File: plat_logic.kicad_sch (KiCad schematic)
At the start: 63 parts, among them SW1 Button-SMD-4.5x4.5x5.5, SW2 Button-SMD-4.5x4.5x5.5, U2 USBLC6-2SC6, U2.1 STM32F429ZIT6TR_split, U2.2 STM32F429ZIT6TR_split, U2.3 STM32F429ZIT6TR_split, U2.4 STM32F429ZIT6TR_split, X1 NX3225GD 8.000MHZ EXS00A-CG06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, X2 NX3215SA-32.768KHZ-EXS00A-MU0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

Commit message: footprints, symbols kicad
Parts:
- removed C1: 2pF, symbol 0805_C9900012713_2
- removed C2: 2pF, symbol 0805_C9900012713_3
- removed C3: 2pF, symbol 0805_C9900012713
- removed C39, C40: 50pF, symbol Device:C
- removed C4: 2pF, symbol 0805_C9900012713_1
- removed C5, C61: 100nF, symbol 0805_C9900012713_6
- removed C6: 1uF x5r, symbol C_0603_US
- removed C7: 2.2uF_x7r, symbol 0805_C9900012713_5
- removed C8: 2.2uF_x7r, symbol 0805_C9900012713_4
- removed Con1: (no value), symbol MyLIB:Con
- removed D26: BAS70, symbol SS54L_19
- removed JP1, JP2: Jumper_2_Open, symbol Jumper:Jumper_2_Open
- removed L1: 1m, symbol L0603_US
- removed R1: 0Ω, symbol RMC1/8JPTP
- removed R10: 0, symbol R_0603_EU_3
- removed R2: 0Ω, symbol RMC1/8JPTP_1
- removed R3: 0, symbol R_0603_EU_6
- removed R39, R41: 25K, symbol Device:R
- removed R4: 0, symbol R_0603_EU_1
- removed R40: 10K, symbol Device:R
- removed R45: 1k, symbol Device:R
- removed R5: 0, symbol R_0603_EU_5
- removed R6: 0, symbol R_0603_EU_4
- removed R63, R64, R65, R66: 2.2k, symbol Device:R
- removed R7: 0, symbol R_0603_EU
- removed R8: 10K, symbol R_0603_EU_7
- removed R9: 0, symbol R_0603_EU_2
- removed SW1, SW2: Button-SMD-4.5x4.5x5.5, symbol Button-SMD-4.5x4.5x5.5
- removed U2: USBLC6-2SC6, Package_TO_SOT_SMD:SOT-23-6, symbol Power_Protection:USBLC6-2SC6
- removed U2.1: STM32F429ZIT6TR_split, symbol STM32F429ZIT6TR_split
- removed U2.2: STM32F429ZIT6TR_split, symbol STM32F429ZIT6TR_split_1
- removed U2.3: STM32F429ZIT6TR_split, symbol STM32F429ZIT6TR_split_2
- removed U2.4: STM32F429ZIT6TR_split, symbol STM32F429ZIT6TR_split_3
- removed X1: NX3225GD 8.000MHZ EXS00A-CG06684, symbol NX3225GD 8.000MHZ EXS00A-CG06684
- removed X2: NX3215SA-32.768KHZ-EXS00A-MU00746, symbol NX3215SA-32.768KHZ-EXS00A-MU00746
- added C10: 1uF_x7r, Capacitor_SMD:C_0603_1608Metric, symbol 0805_C9900012713_5
- added C11: 1uF_x7r, Capacitor_SMD:C_0603_1608Metric, symbol 0805_C9900012713_4
- added C12, C62: 100nF, Capacitor_SMD:C_0402_1005Metric, symbol 0805_C9900012713_6
- added C13: 12pF, Capacitor_SMD:C_0603_1608Metric, symbol 0805_C9900012713_2
- added C14: 12pF, Capacitor_SMD:C_0603_1608Metric, symbol 0805_C9900012713_3
- added C15: 12pF, Capacitor_SMD:C_0603_1608Metric, symbol 0805_C9900012713
- added C16: 12pF, Capacitor_SMD:C_0603_1608Metric, symbol 0805_C9900012713_1
- added C45, C46: 22pF, Capacitor_SMD:C_0603_1608Metric, symbol Device:C
- added C9: 1uF x5r, Capacitor_SMD:C_0603_1608Metric, symbol C_0603_US
- added D28: BAS70, Package_TO_SOT_SMD:SOT-23, symbol SS54L_19
- added JP3, JP4: Jumper_2_Open, Jumper:SolderJumper-2_P1.3mm_Open_Pad1.0x1.5mm, symbol Jumper:Jumper_2_Open
- added L2: 1m, symbol L0603_US
- added R14: 0, symbol R_0603_EU
- added R15: 0, symbol R_0603_EU_1
- added R16: 0, symbol R_0603_EU_6
- added R17: 0, symbol R_0603_EU_5
- added R18: 0, symbol R_0603_EU_4
- added R19: 0, symbol R_0603_EU_2
- added R20: 0, symbol R_0603_EU_3
- added R21: 10K, Resistor_SMD:R_0201_0603Metric, symbol R_0603_EU_7
- added R22: 0Ω, symbol RMC1/8JPTP
- added R35: 0Ω, symbol RMC1/8JPTP_1
- added R49: 1k, Resistor_SMD:R_0805_2012Metric, symbol Device:R
- added R50, R57: 27K, Resistor_SMD:R_0805_2012Metric, symbol Device:R
- added R58: 10K, Resistor_SMD:R_0201_0603Metric, symbol Device:R
- added R67, R68, R69, R70: 2.2k, Resistor_SMD:R_0805_2012Metric, symbol Device:R
- added SW3, SW4: Button-SMD-4.5x4.5x5.5, Button_Switch_SMD:SW_SPST_PTS647_Sx50, symbol Button-SMD-4.5x4.5x5.5
- added U1: STM32F429ZITx, Package_QFP:LQFP-144_20x20mm_P0.5mm, symbol MCU_ST_STM32F4:STM32F429ZITx
- added U3: USBLC6-2SC6, Package_TO_SOT_SMD:SOT-23-6, symbol Power_Protection:USBLC6-2SC6
- added X3: NX3225GD 8.000MHZ EXS00A-CG06684, Crystal:Crystal_SMD_3225-4Pin_3.2x2.5mm, symbol NX3225GD 8.000MHZ EXS00A-CG06684
- added X4: NX3215SA-32.768KHZ-EXS00A-MU00746, Crystal:Crystal_SMD_3215-2Pin_3.2x1.5mm, symbol NX3215SA-32.768KHZ-EXS00A-MU00746
- C42: footprint (none) -> Capacitor_SMD:C_0603_1608Metric
- C47, C48, C49, C50, C51, C52: footprint (none) -> Capacitor_SMD:C_0402_1005Metric
- D27: footprint (none) -> Package_SO:VSSOP-8_2.3x2mm_P0.5mm
- R11: footprint (none) -> Resistor_SMD:R_0805_2012Metric
- R46, R47, R48: footprint (none) -> Resistor_SMD:R_0201_0603Metric
- R51, R52, R53, R54, R55, R56: value 50 -> 47; footprint (none) -> Resistor_SMD:R_0805_2012Metric
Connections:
- net +3v3: now also D28.1 (K), JP3.2 (B), JP4.1 (A), L2.1, R15.1, R18.1, R19.2, R58.2, R67.1, R68.1, R69.1, R70.1, U1.108 (VDD), U1.121 (VDD), U1.131 (VDD), U1.144 (VDD), U1.17 (VDD), U1.30 (VDD), U1.39 (VDD), U1.52 (VDD), U1.62 (VDD), U1.72 (VDD), U1.84 (VDD), U1.95 (VDD)
- net +5v: now also U3.5 (VBUS)
- net A0: now also U1.141 (PE0)
- net A1: now also U1.142 (PE1)
- net A2: now also U1.1 (PE2)
- net A3: now also U1.2 (PE3)
- net A4: now also U1.3 (PE4)
- net A5: now also U1.4 (PE5)
- net A6: now also U1.5 (PE6)
- net A7: now also U1.63 (PE10)
- net AGND: now also U1.31 (VSSA)
- net BOOT0: now also JP3.1 (A), R21.1, U1.138 (BOOT0)
- net BOOT1: now also JP4.2 (B), U1.48 (PB2)
- net D10: now also U1.77 (PD8)
- net D11: now also U1.79 (PD10)
- net D12: now also U1.80 (PD11)
- net D13: now also U1.135 (PB5)
- net D2: now also U1.114 (PD0)
- net D3: now also U1.115 (PD1)
- net D4: now also U1.116 (PD2)
- net D5: now also U1.117 (PD3)
- net D6: now also U1.118 (PD4)
- net D7: now also U1.119 (PD5)
- net D8: now also U1.122 (PD6)
- net D9: now also U1.123 (PD7)
- net DAC(PA4): now also C45.1, R50.1, U1.40 (PA4)
- net DAC(PA5): now also C46.1, R57.1, U1.41 (PA5)
- net ENC_A_M1: now also U1.55 (PF15)
- net ENC_A_M2: now also U1.53 (PF13)
- net ENC_A_M3: now also U1.59 (PE8)
- net ENC_A_M4: now also U1.57 (PG1)
- net ENC_A_M5: now also R67.2, U1.96 (PC6)
- net ENC_A_M6: now also R69.2, U1.81 (PD12)
- net ENC_B_M1: now also U1.56 (PG0)
- net ENC_B_M2: now also U1.54 (PF14)
- net ENC_B_M3: now also U1.60 (PE9)
- net ENC_B_M4: now also U1.58 (PE7)
- net ENC_B_M5: now also R68.2, U1.97 (PC7)
- net ENC_B_M6: now also R70.2, U1.82 (PD13)
- net GND: now also C10.2, C11.1, C12.2, C13.1, C14.1, C15.2, C16.2, C45.2, C46.2, C62.2, C9.2, R16.2, R20.2, R21.2, R50.2, R57.2, SW3.3, SW3.4, SW4.3, SW4.4, U1.107 (VSS), U1.120 (VSS), U1.130 (VSS), U1.16 (VSS), U1.38 (VSS), U1.51 (VSS), U1.61 (VSS), U1.83 (VSS), U1.94 (VSS), U3.2 (GND)
- net I2C2_SCL: now also U1.11 (PF1)
- net I2C2_SDA: now also U1.10 (PF0)
- net I2C_SCL: now also U1.139 (PB8)
- net I2C_SDA: now also U1.140 (PB9)
- net NRST: now also D28.2 (A), R58.1, SW4.1, U1.25 (NRST)
- net PA15: now also U1.110 (PA15)
- net PA2: now also U1.36 (PA2)
- net PA3: now also U1.37 (PA3)
- net PA6: now also U1.42 (PA6)
- net PA7: now also U1.43 (PA7)
- net PC0: now also U1.26 (PC0)
- net PC1: now also U1.27 (PC1)
- net PC3(A2): now also U1.29 (PC3)
- net PF10(A5): now also U1.22 (PF10)
- net PF3(A3): now also U1.13 (PF3)
- net PF5(A4): now also U1.15 (PF5)
- net PG13: now also U1.128 (PG13)
- net PG14: now also U1.129 (PG14)
- net PH2: now also R17.1
- net SWO: now also U1.133 (PB3)
- net TCK: now also U1.109 (PA14)
- net TMS: now also U1.105 (PA13)
- net TX_Enable(Dynamixel_TTL): now also U1.113 (PC12)
- net USART4_RX(Dynamixel_TTL): now also U1.112 (PC11)
- net USART4_TX: now also U1.34 (PA0)
- net USART4_TX(Dynamixel_TTL): now also U1.111 (PC10)
- net VBUS(PA9): now also R49.2
- net ext_RXD: now also U1.69 (PB10)
- net ext_TXD: now also U1.78 (PD9)
- net extra1_enc_A: now also U1.85 (PD14)
- net extra1_enc_B: now also U1.86 (PD15)
- net extra2_enc_A: now also U1.87 (PG2)
- net extra2_enc_B: now also U1.88 (PG3)
- new net: R49.1, U1.101 (PA9)
- new net: U1.103 (PA11), U3.3 (I/O2)
- new net: U1.104 (PA12), U3.1 (I/O1)
- new net: C11.2, R17.2, R18.2, U1.106 (VCAP_2)
- new net: SW3.1, U1.127 (PG12)
- new net: R19.1, R20.1, U1.143 (PDR_ON)
- new net: C9.1, R15.2, U1.6 (VBAT)
- new net: C10.1, R16.1, U1.71 (VCAP_1)
- new net: C13.2, R22.1, X3.1
- new net: C14.2, R35.1, X3.2 (GND)
- new net: L2.2, R14.1
- new net: C12.1, SW4.2
- new net: C62.1, SW3.2
- new net PC14: C15.1, U1.8 (PC14), X4.1 (OSC1)
- new net PC15: C16.1, U1.9 (PC15), X4.2 (OSC2)
- new net PH0: R22.2, U1.23 (PH0)
- new net PH1: R35.2, U1.24 (PH1)
- new net USBDM(PA12): U3.6 (I/O1)
- new net USBDP(PA11): U3.4 (I/O2)
- new net VDDA: R14.2, U1.32 (VREF+), U1.33 (VDDA)
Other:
- moved on the sheet: C42, C47, C48, C49, C50, C51, C52, D27, R11, R12, R13, R46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

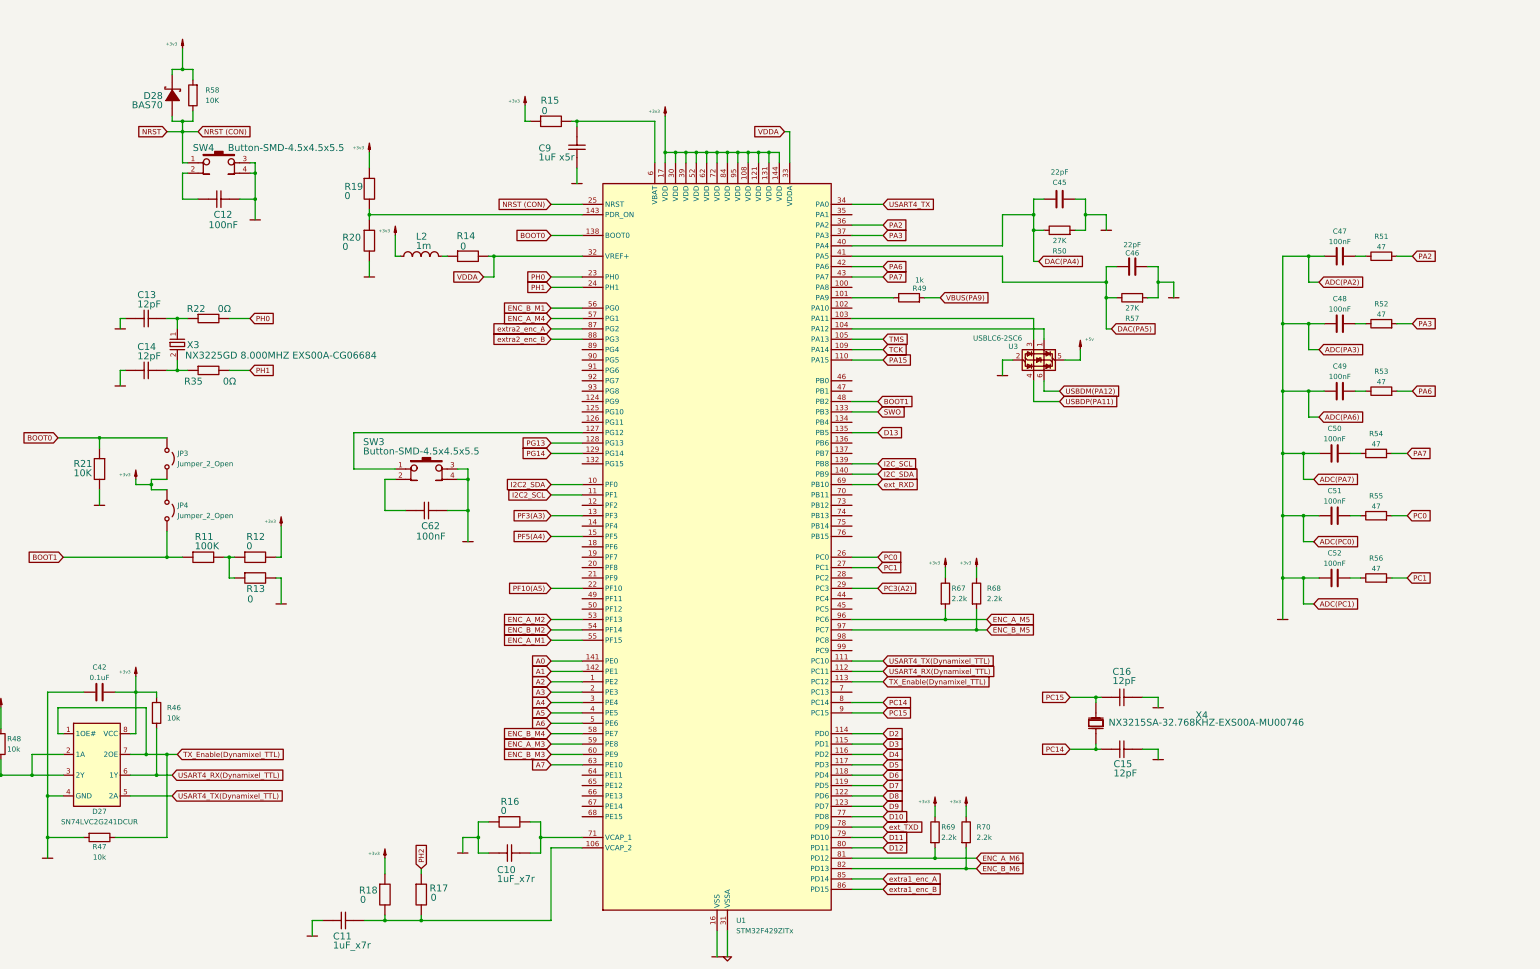
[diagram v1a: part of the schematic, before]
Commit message: Add files via upload
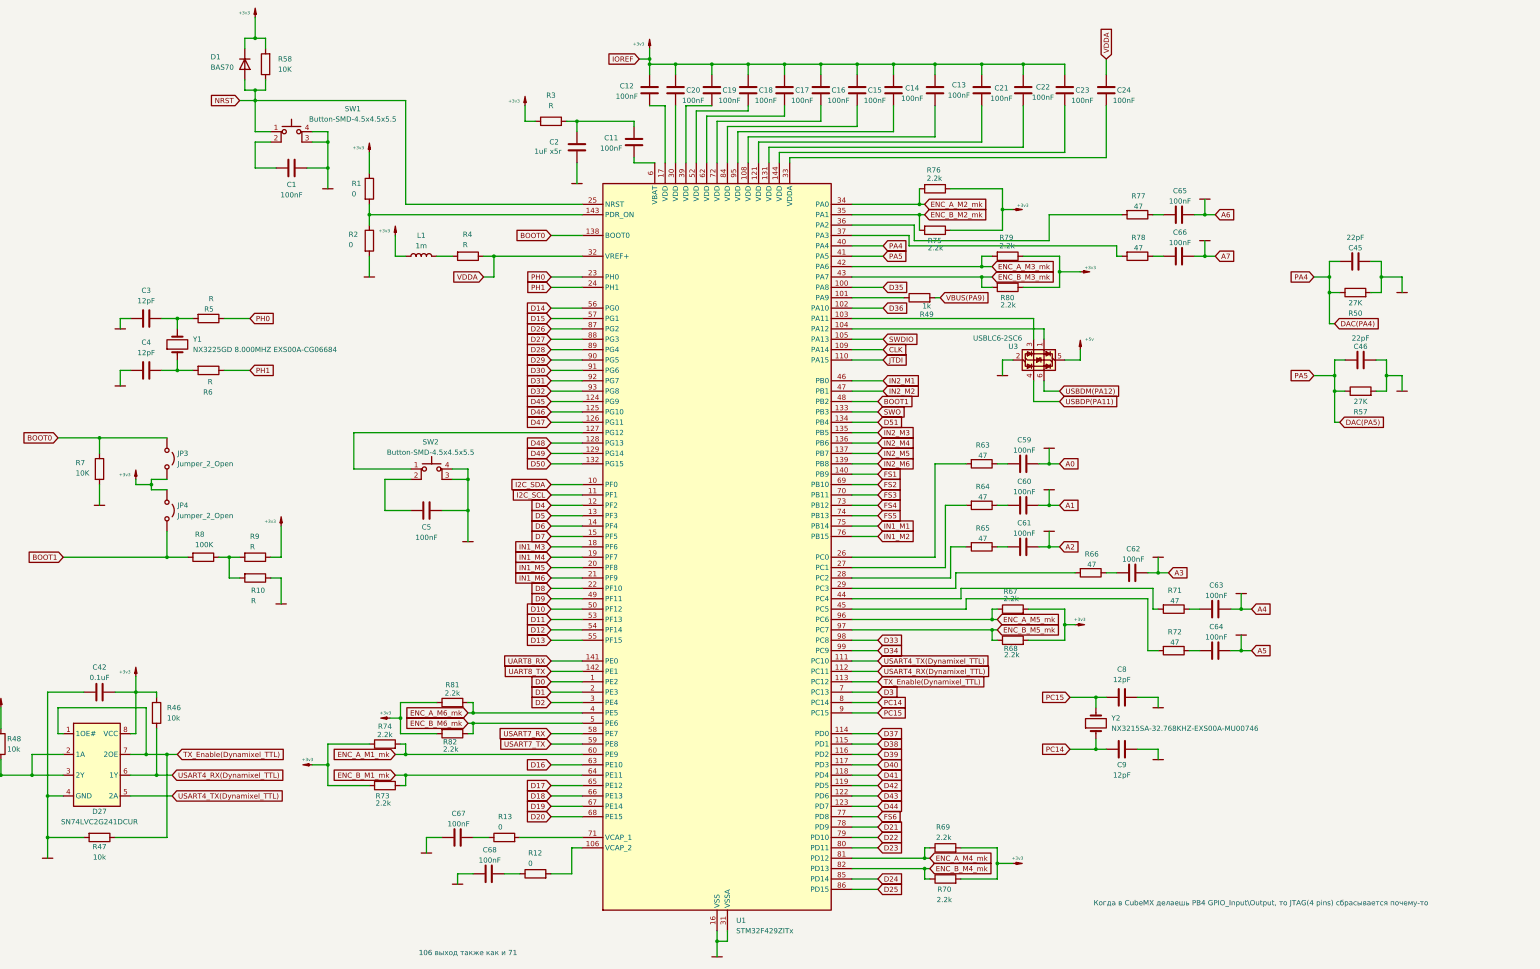
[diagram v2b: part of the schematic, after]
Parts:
- removed C10: 1uF_x7r, Capacitor_SMD:C_0603_1608Metric, symbol 0805_C9900012713_5
- removed C11: 1uF_x7r, Capacitor_SMD:C_0603_1608Metric, symbol 0805_C9900012713_4
- removed C12, C62: 100nF, Capacitor_SMD:C_0402_1005Metric, symbol 0805_C9900012713_6
- removed C13: 12pF, Capacitor_SMD:C_0603_1608Metric, symbol 0805_C9900012713_2
- removed C14: 12pF, Capacitor_SMD:C_0603_1608Metric, symbol 0805_C9900012713_3
- removed C15: 12pF, Capacitor_SMD:C_0603_1608Metric, symbol 0805_C9900012713
- removed C16: 12pF, Capacitor_SMD:C_0603_1608Metric, symbol 0805_C9900012713_1
- removed C47, C48, C49, C50, C51, C52: 100nF, Capacitor_SMD:C_0402_1005Metric, symbol Device:C
- removed C9: 1uF x5r, Capacitor_SMD:C_0603_1608Metric, symbol C_0603_US
- removed D28: BAS70, Package_TO_SOT_SMD:SOT-23, symbol SS54L_19
- removed L2: 1m, symbol L0603_US
- removed R11: 100K, Resistor_SMD:R_0805_2012Metric, symbol R_0603_EU_8
- removed R12: 0, symbol R_0603_EU_9
- removed R13: 0, symbol R_0603_EU_10
- removed R14: 0, symbol R_0603_EU
- removed R15: 0, symbol R_0603_EU_1
- removed R16: 0, symbol R_0603_EU_6
- removed R17: 0, symbol R_0603_EU_5
- removed R18: 0, symbol R_0603_EU_4
- removed R19: 0, symbol R_0603_EU_2
- removed R20: 0, symbol R_0603_EU_3
- removed R21: 10K, Resistor_SMD:R_0201_0603Metric, symbol R_0603_EU_7
- removed R22: 0Ω, symbol RMC1/8JPTP
- removed R35: 0Ω, symbol RMC1/8JPTP_1
- removed R51, R52, R53, R54, R55, R56: 47, Resistor_SMD:R_0805_2012Metric, symbol Device:R
- removed SW3, SW4: Button-SMD-4.5x4.5x5.5, Button_Switch_SMD:SW_SPST_PTS647_Sx50, symbol Button-SMD-4.5x4.5x5.5
- removed X3: NX3225GD 8.000MHZ EXS00A-CG06684, Crystal:Crystal_SMD_3225-4Pin_3.2x2.5mm, symbol NX3225GD 8.000MHZ EXS00A-CG06684
- removed X4: NX3215SA-32.768KHZ-EXS00A-MU00746, Crystal:Crystal_SMD_3215-2Pin_3.2x1.5mm, symbol NX3215SA-32.768KHZ-EXS00A-MU00746
- added C1, C11, C12, C13, C14, C15, C16, C17, C18, C19, C20, C21, C22, C23, C24: 100nF, Capacitor_SMD:C_0603_1608Metric, symbol Device:C
- added C2: 1uF x5r, Capacitor_SMD:C_0603_1608Metric, symbol Device:C
- added C3, C4, C8, C9: 12pF, Capacitor_SMD:C_0603_1608Metric, symbol Device:C
- added C5, C59, C60, C61, C62, C63, C64, C65, C66, C67, C68: 100nF, Capacitor_SMD:C_0402_1005Metric, symbol Device:C
- added D1: BAS70, Diode_SMD:D_0603_1608Metric, symbol Diode:1N914
- added L1: 1m, symbol Device:L
- added R1, R12, R13, R2: 0, Resistor_SMD:R_0805_2012Metric, symbol Device:R
- added R10, R3, R4, R5, R6, R9: R, symbol Device:R
- added R63, R64, R65, R66, R71, R72, R77, R78: 47, Resistor_SMD:R_0805_2012Metric, symbol Device:R
- added R7: 10K, Resistor_SMD:R_0201_0603Metric, symbol Device:R
- added R73, R74, R75, R76, R79, R80, R81, R82: 2.2k, Resistor_SMD:R_0805_2012Metric, symbol Device:R
- added R8: 100K, Resistor_SMD:R_0805_2012Metric, symbol Device:R
- added SW1, SW2: Button-SMD-4.5x4.5x5.5, Button_Switch_SMD:SW_SPST_PTS647_Sx50, symbol Switch:SW_MEC_5E
- added Y1: NX3225GD 8.000MHZ EXS00A-CG06684, Crystal:Crystal_SMD_3225-4Pin_3.2x2.5mm, symbol Device:Crystal
- added Y2: NX3215SA-32.768KHZ-EXS00A-MU00746, Crystal:Crystal_SMD_3215-2Pin_3.2x1.5mm, symbol Device:Crystal
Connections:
- net A4 is gone; now on net D2: U1.3 (PE4)
- net AGND is gone; now on net GND: U1.31 (VSSA)
- net ENC_A_M1 is gone; now on net D13: U1.55 (PF15)
- net ENC_A_M2 is gone; now on net D11: U1.53 (PF13)
- net ENC_B_M2 is gone; now on net D12: U1.54 (PF14)
- net I2C2_SCL is gone; now on net I2C_SCL: U1.11 (PF1)
- net I2C2_SDA is gone; now on net I2C_SDA: U1.10 (PF0)
- net PF10(A5) is gone; now on net D8: U1.22 (PF10)
- net PF3(A3) is gone; now on net D5: U1.13 (PF3)
- net PF5(A4) is gone; now on net D7: U1.15 (PF5)
- net +3v3: now also R67.2, R68.2, R69.2, R70.2, C12.1, C13.1, C14.1, C15.1, C16.1, C17.1, C18.1, C19.1, C20.1, C21.1, C22.1, C23.1, D1.1 (K), L1.1, R1.1, R3.1, R73.2, R74.1, R75.1, R76.1, R79.1, R80.1, R81.1, R82.2, R9.1; no longer R67.1, R68.1, R69.1, R70.1, U1.108 (VDD), U1.121 (VDD), U1.131 (VDD), U1.144 (VDD), U1.17 (VDD), U1.30 (VDD), U1.39 (VDD), U1.52 (VDD), U1.62 (VDD), U1.72 (VDD), U1.84 (VDD), U1.95 (VDD)
- net BOOT0: now also R7.1
- net BOOT1: now also R8.2
- net D10: now also U1.50 (PF12); no longer U1.77 (PD8)
- net D11: no longer U1.79 (PD10)
- net D12: no longer U1.80 (PD11)
- net D13: no longer U1.135 (PB5)
- net D2: no longer U1.114 (PD0)
- net D3: now also U1.7 (PC13); no longer U1.115 (PD1)
- net D4: now also U1.12 (PF2); no longer U1.116 (PD2)
- net D5: no longer U1.117 (PD3)
- net D6: now also U1.14 (PF4); no longer U1.118 (PD4)
- net D7: no longer U1.119 (PD5)
- net D8: no longer U1.122 (PD6)
- net D9: now also U1.49 (PF11); no longer U1.123 (PD7)
- net GND: now also C1.2, C2.1, C3.1, C4.1, C5.2, C59.2, C60.2, C61.2, C62.2, C63.2, C64.2, C65.2, C66.2, C67.1, C68.1, C8.2, C9.2, R10.1, R2.2, R7.2, SW1.3 (K), SW1.4 (A), SW2.3 (K), SW2.4 (A)
- net I2C_SCL: no longer U1.139 (PB8)
- net I2C_SDA: no longer U1.140 (PB9)
- net NRST: now also D1.2 (A), SW1.1
- net PC14: now also C9.1, Y2.1
- net PC15: now also C8.1, Y2.2
- net PH0: now also R5.1
- net PH1: now also R6.1
- net VDDA: now also C24.1, R4.1; no longer U1.33 (VDDA)
- net D35: now reaches U1.100 (PA8)
- net D36: now reaches U1.102 (PA10)
- net at U1.106 (VCAP_2): now also R12.2
- net D45: now reaches U1.124 (PG9)
- net D46: now reaches U1.125 (PG10)
- net D47: now reaches U1.126 (PG11)
- net at U1.127 (PG12): now also SW2.1
- net D50: now reaches U1.132 (PG15)
- net D51: now reaches U1.134 (PB4)
- net IN2_M4: now reaches U1.136 (PB6)
- net IN2_M5: now reaches U1.137 (PB7)
- net at U1.143 (PDR_ON): now also R1.2, R2.1
- net IN1_M3: now reaches U1.18 (PF6)
- net IN1_M4: now reaches U1.19 (PF7)
- net IN1_M5: now reaches U1.20 (PF8)
- net IN1_M6: now reaches U1.21 (PF9)
- net at U1.28 (PC2): now also R65.2
- net ENC_B_M2_mk: now reaches U1.35 (PA1)
- net ENC_B_M2_mk: now also R75.2
- net at U1.44 (PC4): now also R71.2
- net at U1.45 (PC5): now also R72.2
- net IN2_M1: now reaches U1.46 (PB0)
- net IN2_M2: now reaches U1.47 (PB1)
- net at U1.6 (VBAT): now also C11.2
- net ENC_B_M1_mk: now reaches U1.64 (PE11)
- net ENC_B_M1_mk: now also R73.1
- net D17: now reaches U1.65 (PE12)
- net D18: now reaches U1.66 (PE13)
- net D19: now reaches U1.67 (PE14)
- net D20: now reaches U1.68 (PE15)
- net FS3: now reaches U1.70 (PB11)
- net at U1.71 (VCAP_1): now also R13.2
- net FS4: now reaches U1.73 (PB12)
- net FS5: now reaches U1.74 (PB13)
- net IN1_M1: now reaches U1.75 (PB14)
- net IN1_M2: now reaches U1.76 (PB15)
- net D28: now reaches U1.89 (PG4)
- net D29: now reaches U1.90 (PG5)
- net D30: now reaches U1.91 (PG6)
- net D31: now reaches U1.92 (PG7)
- net D32: now reaches U1.93 (PG8)
- net D33: now reaches U1.98 (PC8)
- net D34: now reaches U1.99 (PC9)
- net A0 renamed UART8_RX
- net A1 renamed UART8_TX
- net A2 renamed D0
- net A3 renamed D1
- net A5 renamed ENC_A_M6_mk
- net ENC_A_M6_mk: now also R81.2
- net A6 renamed ENC_B_M6_mk
- net ENC_B_M6_mk: now also R82.1
- net A7 renamed D16
- net ENC_A_M3 renamed USART7_TX
- net ENC_A_M4 renamed D15
- net ENC_A_M5 renamed ENC_A_M5_mk
- net ENC_A_M5_mk: now also R67.1; no longer R67.2
- net ENC_A_M6 renamed ENC_A_M4_mk
- net ENC_A_M4_mk: now also R69.1; no longer R69.2
- net ENC_B_M1 renamed D14
- net ENC_B_M3 renamed ENC_A_M1_mk
- net ENC_A_M1_mk: now also R74.2
- net ENC_B_M4 renamed USART7_RX
- net ENC_B_M5 renamed ENC_B_M5_mk
- net ENC_B_M5_mk: now also R68.1; no longer R68.2
- net ENC_B_M6 renamed ENC_B_M4_mk
- net ENC_B_M4_mk: now also R70.1; no longer R70.2
- net PA15 renamed JTDI
- net PA2: no longer names the net of U1.36 (PA2)
- net PA2: now also R77.2
- net PA3: no longer names the net of U1.37 (PA3)
- net PA3: now also R78.2
- net PA6 renamed ENC_A_M3_mk
- net ENC_A_M3_mk: now also R79.2
- net PA7 renamed ENC_B_M3_mk
- net ENC_B_M3_mk: now also R80.2
- net PC0: no longer names the net of U1.26 (PC0)
- net PC0: now also R63.2
- net PC1: no longer names the net of U1.27 (PC1)
- net PC1: now also R64.2
- net PC3(A2): no longer names the net of U1.29 (PC3)
- net PC3(A2): now also R66.2
- net PG13 renamed D48
- net PG14 renamed D49
- net TCK renamed CLK
- net TMS renamed SWDIO
- net USART4_TX renamed ENC_A_M2_mk
- net ENC_A_M2_mk: now also R76.2
- net ext_RXD renamed FS2
- net ext_TXD renamed D21
- net extra1_enc_A renamed D24
- net extra1_enc_B renamed D25
- net extra2_enc_A renamed D26
- net extra2_enc_B renamed D27
- new net: C1.1, SW1.2
- new net: C13.2, U1.108 (VDD)
- new net: C21.2, U1.121 (VDD)
- new net: C22.2, U1.131 (VDD)
- new net: C23.2, U1.144 (VDD)
- new net: C12.2, U1.17 (VDD)
- new net: C20.2, U1.30 (VDD)
- new net: C24.2, U1.33 (VDDA)
- new net: C19.2, U1.39 (VDD)
- new net: C18.2, U1.52 (VDD)
- new net: C17.2, U1.62 (VDD)
- new net: C16.2, U1.72 (VDD)
- new net: C15.2, U1.84 (VDD)
- new net: C14.2, U1.95 (VDD)
- new net: C11.1, C2.2, R3.2
- new net: C66.1, R78.1
- new net: C62.1, R66.1
- new net: C68.2, R12.1
- new net: L1.2, R4.2
- new net: C63.1, R71.1
- new net: C5.1, SW2.2
- new net: C65.1, R77.1
- new net: C3.2, R5.2, Y1.2
- new net: C67.2, R13.1
- new net: C59.1, R63.1
- new net: C64.1, R72.1
- new net: C60.1, R64.1
- new net: R10.2, R8.1, R9.2
- new net: C4.2, R6.2, Y1.1
- new net: C61.1, R65.1
- new net D22: U1.79 (PD10)
- new net D23: U1.80 (PD11)
- new net D37: U1.114 (PD0)
- new net D38: U1.115 (PD1)
- new net D39: U1.116 (PD2)
- new net D40: U1.117 (PD3)
- new net D41: U1.118 (PD4)
- new net D42: U1.119 (PD5)
- new net D43: U1.122 (PD6)
- new net D44: U1.123 (PD7)
- new net FS1: U1.140 (PB9)
- new net FS6: U1.77 (PD8)
- new net IN2_M3: U1.135 (PB5)
- new net IN2_M6: U1.139 (PB8)
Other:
- note added: "106 выход также как и 71"
- note added: "Когда в CubeMX делаешь PB4 GPIO_Input\Output, то JTAG(4 pins) сбрасывается почему-то"
- moved on the sheet: C45, C46, R49, R50, R57, R58, R67, R68, R69, R70
